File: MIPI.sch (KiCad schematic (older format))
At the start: 47 parts, among them J1 HR911105A, J9 PJ-3270, U1 AllWinner-S3(FBGA-234), Y1 32.768kHz, Y2 24MHz

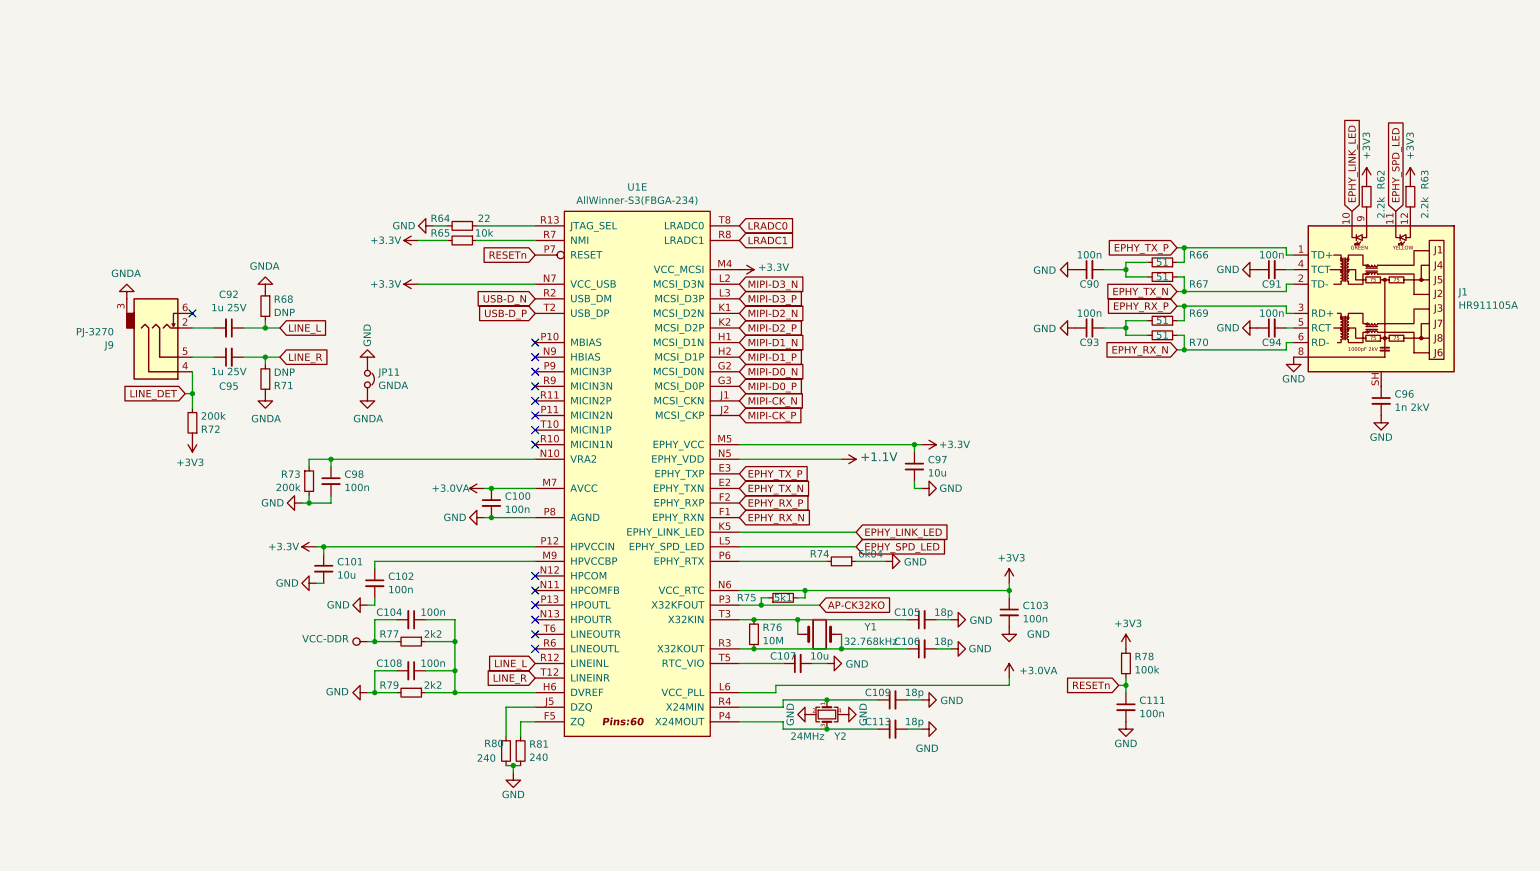
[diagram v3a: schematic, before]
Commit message: V1.0 order release
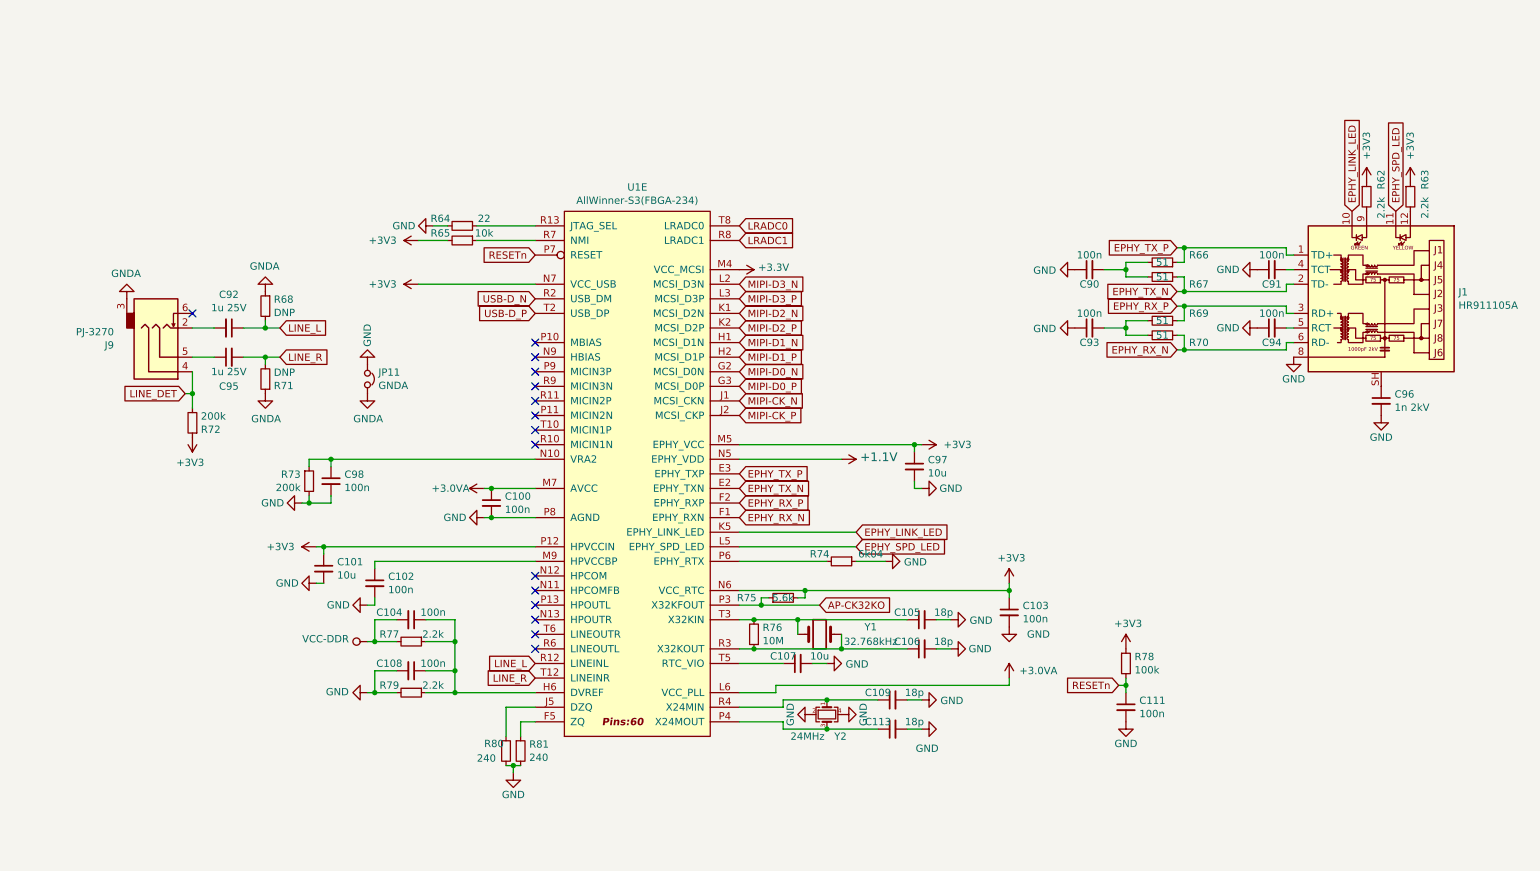
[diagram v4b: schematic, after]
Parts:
- R75: value 5k1 -> 5.6k
- R77, R79: value 2k2 -> 2.2k
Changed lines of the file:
@@
-$EndComp
-$Comp
-L OtterCastAmp-rescue:+3.3V-S3-OLinuXino_Rev_A #PWR?
-U 1 1 621FAA43
-P 3300 2300
-AR Path="/5D8A1FAC/621FAA43" Ref="#PWR?"  Part="1"
-AR Path="/621FAA43" Ref="#PWR?"  Part="1"
-AR Path="/620E795B/621FAA43" Ref="#PWR0165"  Part="1"
-F 0 "#PWR0165" H 3300 2150 50  0001 C CNN
-F 1 "+3.3V" V 3300 2525 50  0000 C CNN
-F 2 "" H 3300 2300 60  0000 C CNN
-F 3 "" H 3300 2300 60  0000 C CNN
-	1    3300 2300
-	0    -1   1    0
 $EndComp
 $Comp
@@
 	1    2950 4500
 	0    1    -1   0
-$EndComp
-$Comp
-L OtterCastAmp-rescue:+3.3V-S3-OLinuXino_Rev_A #PWR?
-U 1 1 621FAAB0
-P 2600 4100
-AR Path="/5D8A1FAC/621FAAB0" Ref="#PWR?"  Part="1"
-AR Path="/621FAAB0" Ref="#PWR?"  Part="1"
-AR Path="/620E795B/621FAAB0" Ref="#PWR0180"  Part="1"
-F 0 "#PWR0180" H 2600 3950 50  0001 C CNN
-F 1 "+3.3V" V 2600 4325 50  0000 C CNN
-F 2 "" H 2600 4100 60  0000 C CNN
-F 3 "" H 2600 4100 60  0000 C CNN
-	1    2600 4100
-	0    -1   1    0
 $EndComp
 $Comp
@@
 	1    6750 3700
 	0    -1   1    0
-$EndComp
-$Comp
-L OtterCastAmp-rescue:+3.3V-S3-OLinuXino_Rev_A #PWR?
-U 1 1 621FABA1
-P 6750 3400
-AR Path="/5D8A1FAC/621FABA1" Ref="#PWR?"  Part="1"
-AR Path="/621FABA1" Ref="#PWR?"  Part="1"
-AR Path="/620E795B/621FABA1" Ref="#PWR0174"  Part="1"
-F 0 "#PWR0174" H 6750 3250 50  0001 C CNN
-F 1 "+3.3V" V 6750 3625 50  0000 C CNN
-F 2 "" H 6750 3400 60  0000 C CNN
-F 3 "" H 6750 3400 60  0000 C CNN
-	1    6750 3400
-	0    1    -1   0
 $EndComp
 $Comp
@@
 AR Path="/620E795B/6859B564" Ref="R77"  Part="1"
 F 0 "R77" V 3200 4600 50  0000 C CNN
-F 1 "2k2" V 3200 4900 50  0000 C CNN
+F 1 "2.2k" V 3200 4900 50  0000 C CNN
 F 2 "otter:R_0402" H 3250 4750 50  0001 C CNN
 F 3 "~" H 3250 4750 50  0001 C CNN
@@
 AR Path="/620E795B/68A2F582" Ref="R75"  Part="1"
 F 0 "R75" V 5800 4700 50  0000 C CNN
-F 1 "5k1" V 5800 4450 50  0000 C CNN
+F 1 "5.6k" V 5800 4450 50  0000 C CNN
 F 2 "otter:R_0402" H 5800 4450 50  0001 C CNN
 F 3 "~" H 5800 4450 50  0001 C CNN
@@
 AR Path="/620E795B/68CF6E99" Ref="R79"  Part="1"
 F 0 "R79" V 3200 4950 50  0000 C CNN
-F 1 "2k2" V 3200 5250 50  0000 C CNN
+F 1 "2.2k" V 3200 5250 50  0000 C CNN
 F 2 "otter:R_0402" H 3250 5100 50  0001 C CNN
 F 3 "~" H 3250 5100 50  0001 C CNN
@@
 Wire Wire Line
 	4100 2000 3700 2000
-$Comp
-L OtterCastAmp-rescue:+3.3V-S3-OLinuXino_Rev_A #PWR?
-U 1 1 6138FD33
-P 3300 2000
-AR Path="/5D8A1FAC/6138FD33" Ref="#PWR?"  Part="1"
-AR Path="/6138FD33" Ref="#PWR?"  Part="1"
-AR Path="/620E795B/6138FD33" Ref="#PWR0161"  Part="1"
-F 0 "#PWR0161" H 3300 1850 50  0001 C CNN
-F 1 "+3.3V" V 3300 2225 50  0000 C CNN
-F 2 "" H 3300 2000 60  0000 C CNN
-F 3 "" H 3300 2000 60  0000 C CNN
-	1    3300 2000
-	0    -1   1    0
-$EndComp
 Wire Wire Line
 	3300 2000 3500 2000
@@
 Wire Wire Line
 	5500 3500 6200 3500
+$Comp
+L power:+3V3 #PWR?
+U 1 1 60456E38
+P 6750 3400
+F 0 "#PWR?" H 6750 3250 50  0001 C CNN
+F 1 "+3V3" V 6750 3550 50  0000 L CNN
+F 2 "" H 6750 3400 50  0001 C CNN
+F 3 "" H 6750 3400 50  0001 C CNN
+	1    6750 3400
+	0    1    1    0
+$EndComp
+$Comp
+L power:+3V3 #PWR?
+U 1 1 6045BE88
+P 3300 2000
+F 0 "#PWR?" H 3300 1850 50  0001 C CNN
+F 1 "+3V3" V 3300 2150 50  0000 L CNN
+F 2 "" H 3300 2000 50  0001 C CNN
+F 3 "" H 3300 2000 50  0001 C CNN
+	1    3300 2000
+	0    -1   -1   0
+$EndComp
+$Comp
+L power:+3V3 #PWR?
+U 1 1 6045C548
+P 3300 2300
+F 0 "#PWR?" H 3300 2150 50  0001 C CNN
+F 1 "+3V3" V 3300 2450 50  0000 L CNN
+F 2 "" H 3300 2300 50  0001 C CNN
+F 3 "" H 3300 2300 50  0001 C CNN
+	1    3300 2300
+	0    -1   -1   0
+$EndComp
+$Comp
+L power:+3V3 #PWR?
+U 1 1 6045CECD
+P 2600 4100
+F 0 "#PWR?" H 2600 3950 50  0001 C CNN
+F 1 "+3V3" V 2600 4250 50  0000 L CNN
+F 2 "" H 2600 4100 50  0001 C CNN
+F 3 "" H 2600 4100 50  0001 C CNN
+	1    2600 4100
+	0    -1   -1   0
+$EndComp
 $EndSCHEMATC

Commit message: cleaned up libs
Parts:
- J1: symbol otter:HR911105A -> OtterCastAmp-rescue:HR911105A-otter
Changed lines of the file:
@@
 $EndComp
 $Comp
-L otter:HR911105A J1
+L OtterCastAmp-rescue:HR911105A-otter J1
 U 1 1 60B1E955
 P 9900 2400

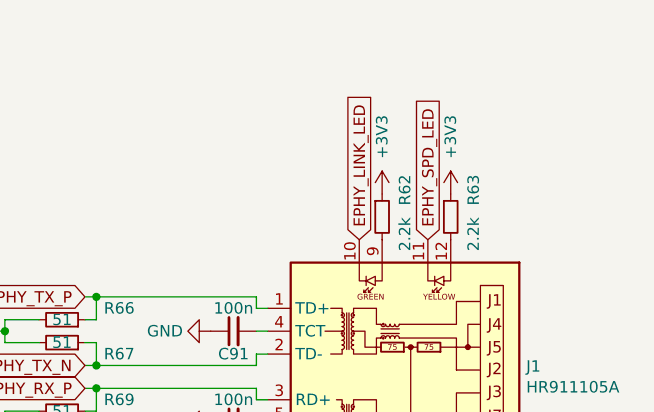
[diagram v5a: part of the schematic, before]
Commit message: V1.2 production release
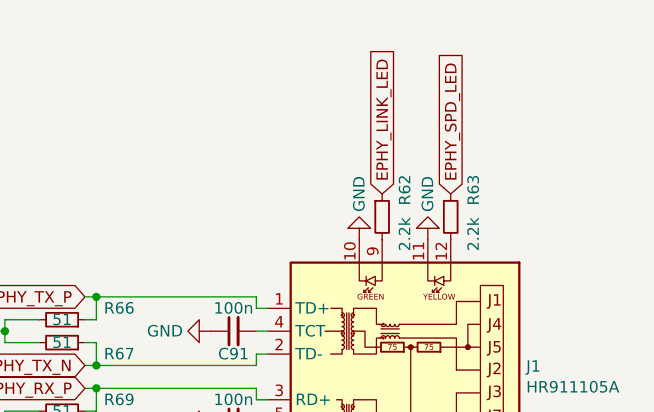
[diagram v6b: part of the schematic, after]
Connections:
- net +3V3: no longer R62.1, R63.1
- net EPHY_LINK_LED: now also R62.1; no longer J1.10
- net EPHY_SPD_LED: now also R63.1; no longer J1.11
- net GND: now also J1.10, J1.11
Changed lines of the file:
@@
 Text GLabel 8500 2750 0    50   Input ~ 0
 EPHY_RX_N
-Text GLabel 9700 1800 1    50   Input ~ 0
+Text GLabel 9800 1600 1    50   Input ~ 0
 EPHY_LINK_LED
 $Comp
@@
 	1750 3050 1750 2900
 $Comp
-L power:+3V3 #PWR0158
-U 1 1 61A2646E
-P 9800 1600
-F 0 "#PWR0158" H 9800 1450 50  0001 C CNN
-F 1 "+3V3" V 9800 1850 50  0000 C CNN
-F 2 "" H 9800 1600 50  0001 C CNN
-F 3 "" H 9800 1600 50  0001 C CNN
-	1    9800 1600
-	1    0    0    -1
-$EndComp
-$Comp
 L Device:R_Small R62
 U 1 1 61A2ACF4
@@
 	1    0    0    -1
 $EndComp
-Text GLabel 10000 1800 1    50   Input ~ 0
+Text GLabel 10100 1600 1    50   Input ~ 0
 EPHY_SPD_LED
-$Comp
-L power:+3V3 #PWR0159
-U 1 1 61A4052D
-P 10100 1600
-F 0 "#PWR0159" H 10100 1450 50  0001 C CNN
-F 1 "+3V3" V 10100 1850 50  0000 C CNN
-F 2 "" H 10100 1600 50  0001 C CNN
-F 3 "" H 10100 1600 50  0001 C CNN
-	1    10100 1600
-	1    0    0    -1
-$EndComp
 $Comp
 L Device:C_Small C?
@@
 	5500 3500 6200 3500
 $Comp
-L power:+3V3 #PWR?
+L power:+3V3 #PWR0174
 U 1 1 60456E38
 P 6750 3400
-F 0 "#PWR?" H 6750 3250 50  0001 C CNN
+F 0 "#PWR0174" H 6750 3250 50  0001 C CNN
 F 1 "+3V3" V 6750 3550 50  0000 L CNN
 F 2 "" H 6750 3400 50  0001 C CNN
@@
 $EndComp
 $Comp
-L power:+3V3 #PWR?
+L power:+3V3 #PWR0178
 U 1 1 6045BE88
 P 3300 2000
-F 0 "#PWR?" H 3300 1850 50  0001 C CNN
+F 0 "#PWR0178" H 3300 1850 50  0001 C CNN
 F 1 "+3V3" V 3300 2150 50  0000 L CNN
 F 2 "" H 3300 2000 50  0001 C CNN
@@
 $EndComp
 $Comp
-L power:+3V3 #PWR?
+L power:+3V3 #PWR0180
 U 1 1 6045C548
 P 3300 2300
-F 0 "#PWR?" H 3300 2150 50  0001 C CNN
+F 0 "#PWR0180" H 3300 2150 50  0001 C CNN
 F 1 "+3V3" V 3300 2450 50  0000 L CNN
 F 2 "" H 3300 2300 50  0001 C CNN
@@
 $EndComp
 $Comp
-L power:+3V3 #PWR?
+L power:+3V3 #PWR0216
 U 1 1 6045CECD
 P 2600 4100
-F 0 "#PWR?" H 2600 3950 50  0001 C CNN
+F 0 "#PWR0216" H 2600 3950 50  0001 C CNN
 F 1 "+3V3" V 2600 4250 50  0000 L CNN
 F 2 "" H 2600 4100 50  0001 C CNN
@@
 	0    -1   -1   0
 $EndComp
+$Comp
+L OtterCastAmp-rescue:GND-S3-OLinuXino_Rev_A #PWR?
+U 1 1 6080D464
+P 9700 1800
+AR Path="/5D8A1FAC/6080D464" Ref="#PWR?"  Part="1"
+AR Path="/6080D464" Ref="#PWR?"  Part="1"
+AR Path="/620E795B/6080D464" Ref="#PWR0158"  Part="1"
+F 0 "#PWR0158" H 9700 1550 50  0001 C CNN
+F 1 "GND" V 9700 1600 50  0000 C CNN
+F 2 "" H 9700 1800 60  0000 C CNN
+F 3 "" H 9700 1800 60  0000 C CNN
+	1    9700 1800
+	-1   0    0    1
+$EndComp
+$Comp
+L OtterCastAmp-rescue:GND-S3-OLinuXino_Rev_A #PWR?
+U 1 1 6080D947
+P 10000 1800
+AR Path="/5D8A1FAC/6080D947" Ref="#PWR?"  Part="1"
+AR Path="/6080D947" Ref="#PWR?"  Part="1"
+AR Path="/620E795B/6080D947" Ref="#PWR0159"  Part="1"
+F 0 "#PWR0159" H 10000 1550 50  0001 C CNN
+F 1 "GND" V 10000 1600 50  0000 C CNN
+F 2 "" H 10000 1800 60  0000 C CNN
+F 3 "" H 10000 1800 60  0000 C CNN
+	1    10000 1800
+	-1   0    0    1
+$EndComp
 $EndSCHEMATC
